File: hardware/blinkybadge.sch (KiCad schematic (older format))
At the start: 23 parts, among them IC101 ATMEGA8U2, P101 USB_OTG, P102 CONN_02X03, Q101 Q_PMOS_GDS, SW101 SPST, U101 ATECC508A, Y101 16MHz

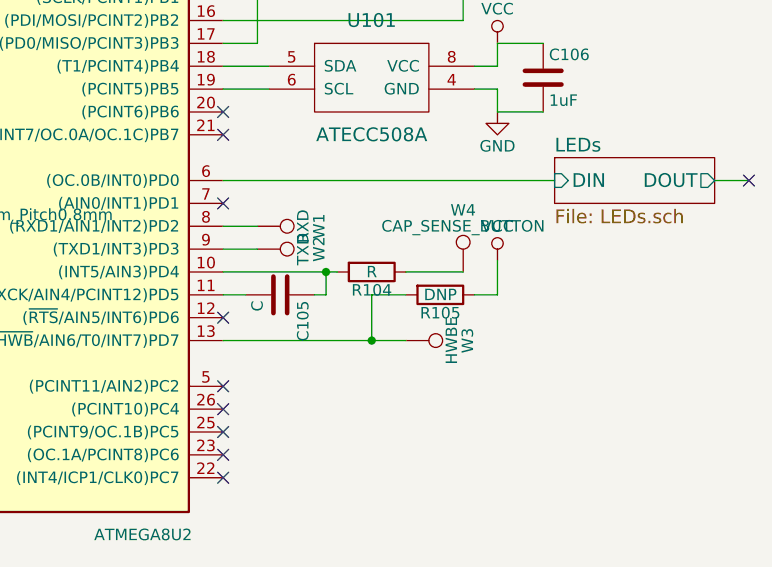
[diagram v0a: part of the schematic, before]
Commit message: Add some layout tweaks
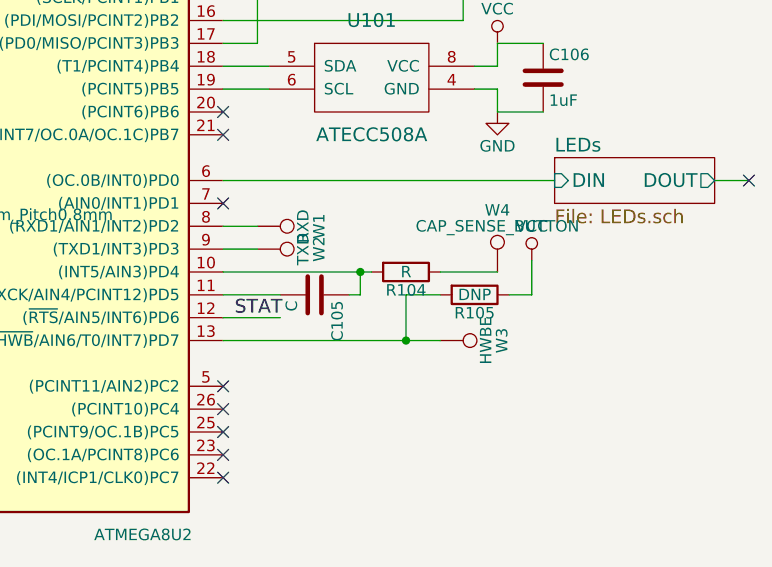
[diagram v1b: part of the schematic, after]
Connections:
- net STAT: now also IC101.12 ((~RTS~/AIN5/INT6)PD6)
- no-connect marks 12 -> 11
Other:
- moved on the sheet: C105, R104, R105, W3, W4
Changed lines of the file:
@@
 L C C105
 U 1 1 577EF93B
-P 7050 4650
-F 0 "C105" H 7075 4750 50  0000 L CNN
-F 1 "C" H 7075 4550 50  0000 L CNN
-F 2 "Capacitors_SMD:C_0603" H 7088 4500 50  0001 C CNN
-F 3 "" H 7050 4650 50  0000 C CNN
-	1    7050 4650
+P 7200 4650
+F 0 "C105" H 7225 4750 50  0000 L CNN
+F 1 "C" H 7225 4550 50  0000 L CNN
+F 2 "Capacitors_SMD:C_0603" H 7238 4500 50  0001 C CNN
+F 3 "" H 7200 4650 50  0000 C CNN
+	1    7200 4650
 	0    1    1    0
 $EndComp
@@
 L R R104
 U 1 1 577EF9C0
-P 7450 4550
-F 0 "R104" V 7530 4550 50  0000 C CNN
-F 1 "R" V 7450 4550 50  0000 C CNN
-F 2 "Resistors_SMD:R_0603" V 7380 4550 50  0001 C CNN
-F 3 "" H 7450 4550 50  0000 C CNN
-	1    7450 4550
+P 7600 4550
+F 0 "R104" V 7680 4550 50  0000 C CNN
+F 1 "R" V 7600 4550 50  0000 C CNN
+F 2 "Resistors_SMD:R_0603" V 7530 4550 50  0001 C CNN
+F 3 "" H 7600 4550 50  0000 C CNN
+	1    7600 4550
 	0    1    1    0
 $EndComp
@@
 	8950 4150 9100 4150
 Wire Wire Line
-	6800 4550 7300 4550
-Wire Wire Line
-	6800 4650 6900 4650
-Wire Wire Line
-	7200 4650 7250 4650
-Wire Wire Line
-	7250 4650 7250 4550
-Connection ~ 7250 4550
-Wire Wire Line
-	7600 4550 7850 4550
+	6800 4550 7450 4550
+Wire Wire Line
+	6800 4650 7050 4650
+Wire Wire Line
+	7350 4650 7400 4650
+Wire Wire Line
+	7400 4650 7400 4550
+Connection ~ 7400 4550
+Wire Wire Line
+	7750 4550 8000 4550
 Wire Wire Line
 	4600 2750 7200 2750
@@
 L TEST_1P W4
 U 1 1 57805F3E
-P 7850 4550
-F 0 "W4" H 7850 4820 50  0000 C CNN
-F 1 "CAP_SENSE_BUTTON" H 7850 4750 50  0000 C CNN
-F 2 "Measurement_Points:Measurement_Point_Round-SMD-Pad_Small" H 8050 4550 50  0001 C CNN
-F 3 "" H 8050 4550 50  0000 C CNN
-	1    7850 4550
+P 8000 4550
+F 0 "W4" H 8000 4820 50  0000 C CNN
+F 1 "CAP_SENSE_BUTTON" H 8000 4750 50  0000 C CNN
+F 2 "Measurement_Points:Measurement_Point_Round-SMD-Pad_Small" H 8200 4550 50  0001 C CNN
+F 3 "" H 8200 4550 50  0000 C CNN
+	1    8000 4550
 	1    0    0    -1
 $EndComp
@@
 L TEST_1P W3
 U 1 1 57845845
-P 7600 4850
-F 0 "W3" H 7600 5120 50  0000 C CNN
-F 1 "HWBE" H 7600 5050 50  0000 C CNN
-F 2 "Measurement_Points:Measurement_Point_Round-SMD-Pad_Small" H 7800 4850 50  0001 C CNN
-F 3 "" H 7800 4850 50  0000 C CNN
-	1    7600 4850
-	0    1    1    0
-$EndComp
-Wire Wire Line
-	6800 4850 7600 4850
+P 7750 4850
+F 0 "W3" H 7750 5120 50  0000 C CNN
+F 1 "HWBE" H 7750 5050 50  0000 C CNN
+F 2 "Measurement_Points:Measurement_Point_Round-SMD-Pad_Small" H 7950 4850 50  0001 C CNN
+F 3 "" H 7950 4850 50  0000 C CNN
+	1    7750 4850
+	0    1    1    0
+$EndComp
+Wire Wire Line
+	6800 4850 7750 4850
 $Comp
 L R R105
 U 1 1 57846CBE
-P 7750 4650
-F 0 "R105" V 7830 4650 50  0000 C CNN
-F 1 "DNP" V 7750 4650 50  0000 C CNN
-F 2 "Resistors_SMD:R_0603" V 7680 4650 50  0001 C CNN
-F 3 "" H 7750 4650 50  0000 C CNN
-	1    7750 4650
-	0    1    1    0
-$EndComp
-Wire Wire Line
-	7600 4650 7450 4650
-Wire Wire Line
-	7450 4650 7450 4850
-Connection ~ 7450 4850
-Wire Wire Line
-	7900 4650 8000 4650
-Wire Wire Line
-	8000 4650 8000 4500
+P 7900 4650
+F 0 "R105" V 7980 4650 50  0000 C CNN
+F 1 "DNP" V 7900 4650 50  0000 C CNN
+F 2 "Resistors_SMD:R_0603" V 7830 4650 50  0001 C CNN
+F 3 "" H 7900 4650 50  0000 C CNN
+	1    7900 4650
+	0    1    1    0
+$EndComp
+Wire Wire Line
+	7750 4650 7600 4650
+Wire Wire Line
+	7600 4650 7600 4850
+Connection ~ 7600 4850
+Wire Wire Line
+	8050 4650 8150 4650
+Wire Wire Line
+	8150 4650 8150 4500
 $Comp
 L VCC #PWR013
 U 1 1 57846ECD
-P 8000 4500
-F 0 "#PWR013" H 8000 4350 50  0001 C CNN
-F 1 "VCC" H 8000 4650 50  0000 C CNN
-F 2 "" H 8000 4500 50  0000 C CNN
-F 3 "" H 8000 4500 50  0000 C CNN
-	1    8000 4500
+P 8150 4500
+F 0 "#PWR013" H 8150 4350 50  0001 C CNN
+F 1 "VCC" H 8150 4650 50  0000 C CNN
+F 2 "" H 8150 4500 50  0000 C CNN
+F 3 "" H 8150 4500 50  0000 C CNN
+	1    8150 4500
 	1    0    0    -1
 $EndComp
@@
 NoConn ~ 6800 5350
 NoConn ~ 6800 5450
-NoConn ~ 6800 4750
 Wire Wire Line
 	7900 3650 8000 3650
 Wire Wire Line
 	5700 1700 5700 2950
+Wire Wire Line
+	6800 4750 7050 4750
+Text Label 6850 4750 0    60   ~ 0
+STAT
 $EndSCHEMATC
